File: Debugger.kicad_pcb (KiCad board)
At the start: 4 copper layers, 66 x 24.3 mm, 33 parts, among them J1 Internal clock, J2 I/O, J3 NAND0, J4 NAND1, Q1 BC546, SW1 Single step, U1 74LS132, U2 NE555P, U3 74LS74

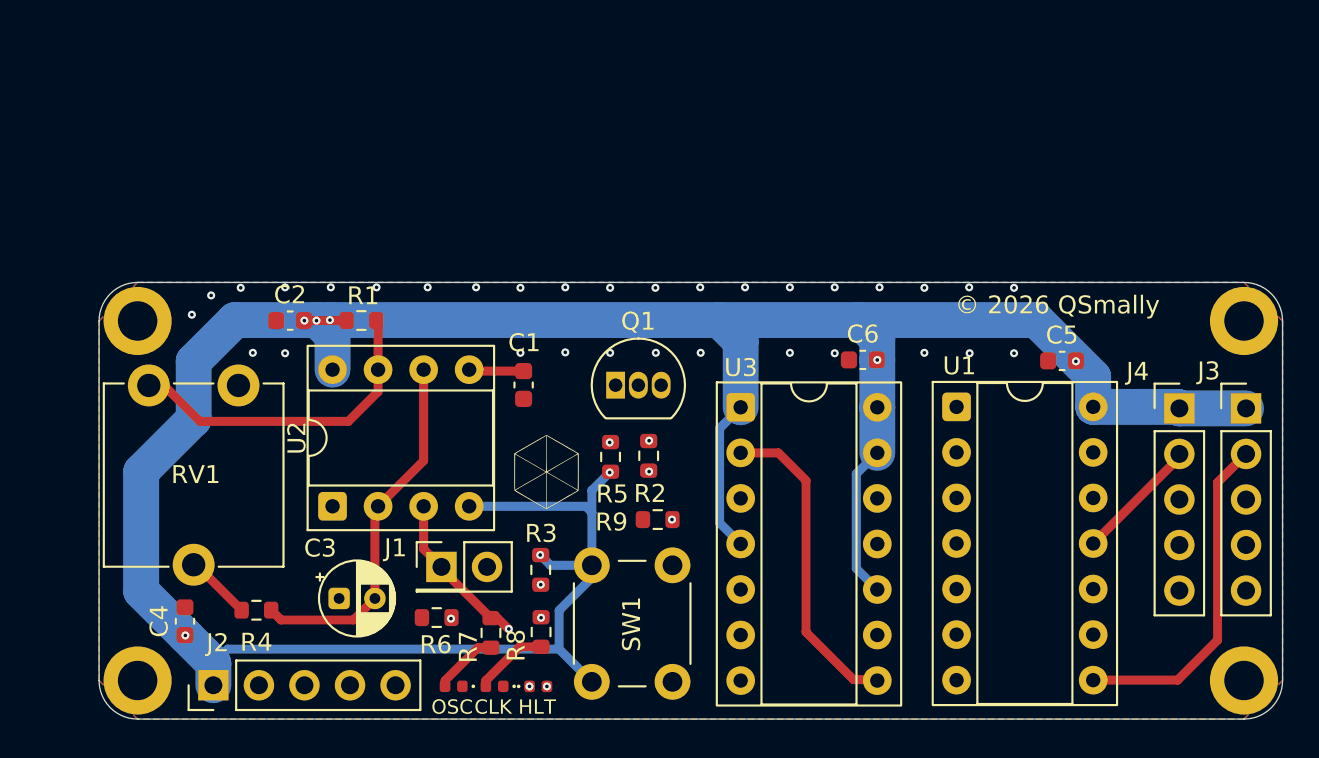
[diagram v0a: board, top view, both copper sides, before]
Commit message: Board: revision 2
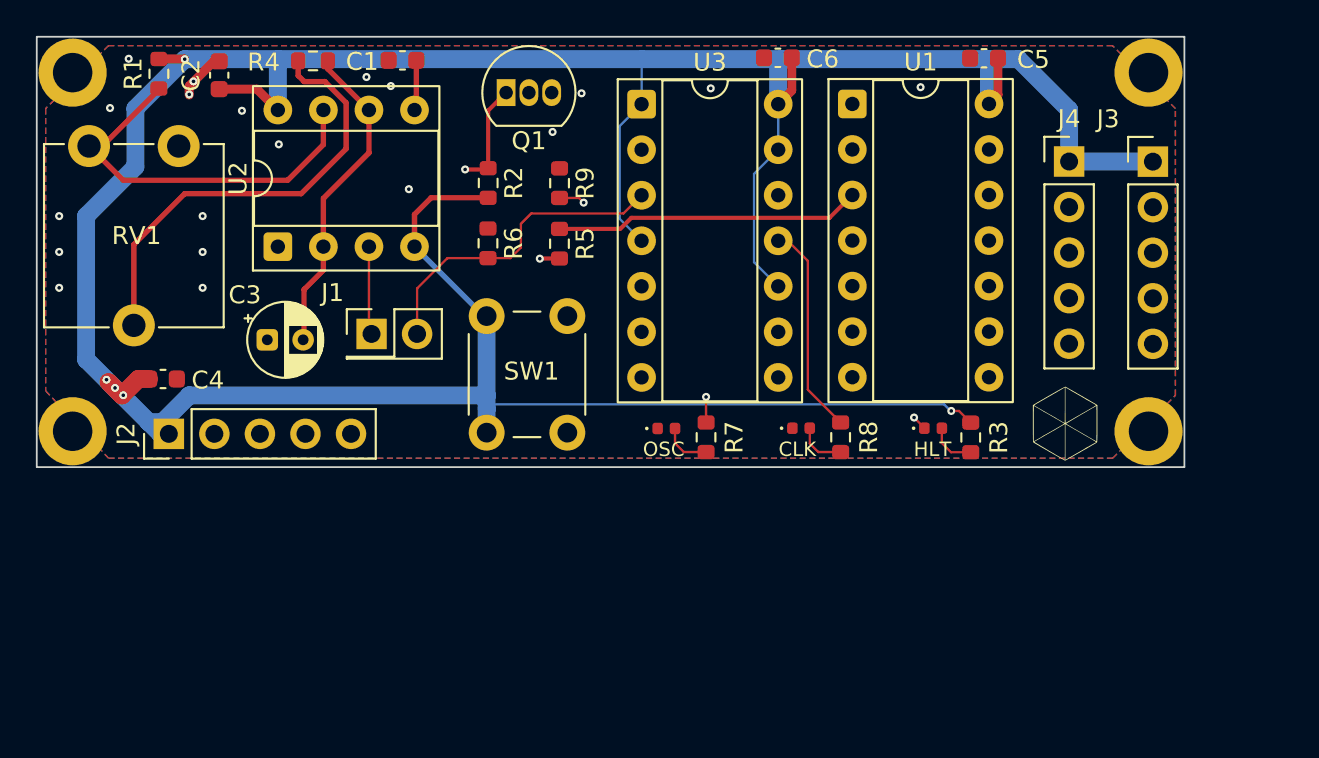
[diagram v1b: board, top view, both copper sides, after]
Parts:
- moved R4 30.8 mm to (113.4, 79.3)
- moved G*** 29.0 mm to (155.3, 99.6)
- moved D1 26.3 mm to (148.0, 99.8)
- moved R3 25.1 mm to (150.1, 100.3)
- moved D3 22.3 mm to (140.6, 99.8), turned to 0 degrees
- moved R6 21.1 mm to (123.2, 89.5), turned to -90 degrees
- moved R8 19.9 mm to (142.8, 100.3)
- moved R9 19.5 mm to (127.2, 86.2), turned to -90 degrees
- moved C1 19.3 mm to (118.4, 79.3), turned to 0 degrees
- moved D2 18.6 mm to (133.1, 99.8), turned to 0 degrees
- moved U1 17.9 mm to (143.5, 81.7)
- moved R1 17.8 mm to (104.8, 80.1), turned to 90 degrees
- moved U3 17.8 mm to (131.7, 81.8)
- moved C6 17.5 mm to (139.3, 79.2)
- moved C5 17.4 mm to (150.8, 79.2)
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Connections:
- J2 pad 2: /OSC -> GND
- J2 pad 3: /CLK -> /OSC
- J2 pad 4: //HALT -> /CLK
- J2 pad 5: GND -> //HALT
- J3 pad 2: Net-(J3-Pin_2) -> GND
- J3 pad 5: GND -> Net-(J3-Pin_5)
- J4 pad 2: Net-(J4-Pin_2) -> GND
- J4 pad 5: GND -> Net-(J4-Pin_5)
- U1 pad 11: Net-(J4-Pin_2) -> Net-(J4-Pin_5)
- U1 pad 8: Net-(J3-Pin_2) -> Net-(J3-Pin_5)
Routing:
- net +5V: track 162.8 -> 193.0 mm, vias 8 -> 5
- net //HALT: track 30.9 -> 58.8 mm
- net Net-(R4-Pad1): track 3.73 -> 25.2 mm
- net Net-(J3-Pin_2): track 18.9 -> 0.00 mm
- net /CLK: track 42.5 -> 54.3 mm, vias 2 -> 0
- net Net-(J3-Pin_5): track 0.00 -> 9.91 mm
- net Net-(J4-Pin_5): track 0.00 -> 9.49 mm
- net Net-(Q1-B): track 3.34 -> 10.6 mm
- net Net-(J4-Pin_2): track 6.99 -> 0.00 mm
- net /OSC: track 42.5 -> 37.0 mm
- net Net-(J1-Pin_1): track 37.6 -> 42.9 mm
- net Net-(D1-A): track 7.39 -> 2.65 mm, vias 2 -> 0
- net /STEP: track 22.0 -> 26.5 mm
- net Net-(U2-DISCH): track 17.8 -> 21.9 mm
- net Net-(J4-Pin_4): track 6.18 -> 9.49 mm
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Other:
- board size 66 x 24.3 mm -> 64 x 24 mm
- board text removed: "© 2026 QSmally"
